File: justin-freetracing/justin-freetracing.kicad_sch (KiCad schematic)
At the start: 114 parts, among them J1 Conn_01x08_MountingPin, J2 Conn_02x03_Odd_Even, J3 Conn_01x08_MountingPin, J5 Barrel_Jack_Switch_Pin3Ring, K1 SW_Push, K10 SW_Push, K11 SW_Push, K12 SW_Push, K13 SW_Push, K14 SW_Push, K15 SW_Push, K16 SW_Push, K17 SW_Push, K18 SW_Push, K19 SW_Push, K2 SW_Push, K20 SW_Push, K21 SW_Push, K22 SW_Push, K23 SW_Push, K24 SW_Push, K25 SW_Push, K26 SW_Push, K27 SW_Push, K28 SW_Push, K29 SW_Push, K3 SW_Push, K30 SW_Push, K31 SW_Push, K32 SW_Push, K33 SW_Push, K34 SW_Push, K35 SW_Push, K36 SW_Push, K37 SW_Push, K38 SW_Push, K39 SW_Push, K4 SW_Push, K40 SW_Push, K41 SW_Push, K42 SW_Push, K43 SW_Push, K44 SW_Push, K45 SW_Push, K46 SW_Push, K47 SW_Push, K48 SW_Push, K49 SW_Push, K5 SW_Push, K6 SW_Push, K7 SW_Push, K8 SW_Push, K9 SW_Push, U1 ATmega1284-P, Y1 20MHz

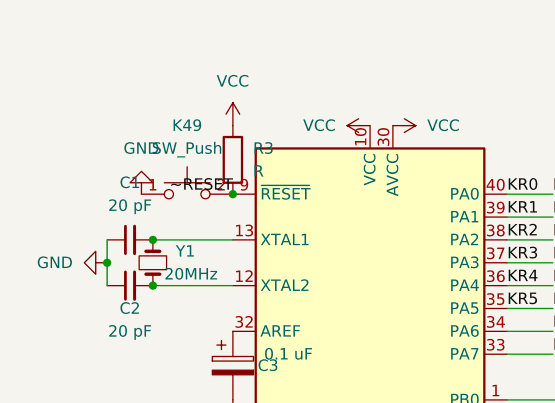
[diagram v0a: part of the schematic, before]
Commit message: Push
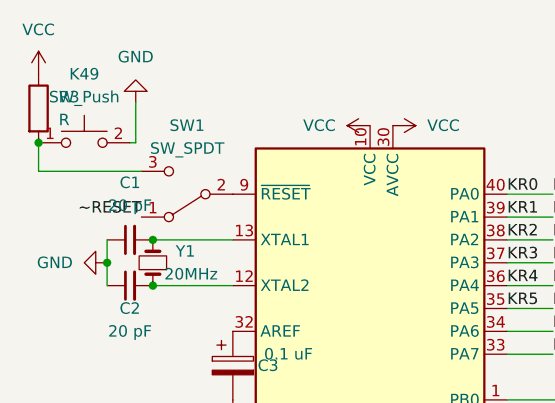
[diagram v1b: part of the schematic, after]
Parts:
- added SW1: SW_SPDT, Connector_PinSocket_2.54mm:PinSocket_1x03_P2.54mm_Vertical, symbol Switch:SW_SPDT
- R1, R2, R3: footprint Resistor_THT:R_Axial_DIN0204_L3.6mm_D1.6mm_P5.08mm_Horizontal -> Resistor_THT:R_Axial_DIN0204_L3.6mm_D1.6mm_P7.62mm_Horizontal
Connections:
- net GND: now also K49.2; no longer K49.1
- net ~RESET: now also SW1.1 (A); no longer K49.2, R3.2, U1.9 (~{RESET})
- new net: SW1.2 (B), U1.9 (~{RESET})
- new net: K49.1, R3.2, SW1.3 (C)
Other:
- moved on the sheet: K49, R3
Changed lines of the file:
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@@
   (junction (at 172.72 66.04) (diameter 0) (color 0 0 0 0)
   )
+  (junction (at 15.24 20.955) (diameter 0) (color 0 0 0 0)
+  )
   (junction (at 209.55 81.28) (diameter 0) (color 0 0 0 0)
   )
@@
   (junction (at 153.67 128.27) (diameter 0) (color 0 0 0 0)
   )
-  (junction (at 36.83 26.67) (diameter 0) (color 0 0 0 0)
-  )
   (junction (at 153.67 102.87) (diameter 0) (color 0 0 0 0)
   )
@@
     (stroke (width 0) (type default) (color 0 0 0 0))
   )
+  (wire (pts (xy 15.24 24.13) (xy 26.67 24.13))
+    (stroke (width 0) (type default) (color 0 0 0 0))
+  )
   (wire (pts (xy 144.78 68.58) (xy 152.4 68.58))
     (stroke (width 0) (type default) (color 0 0 0 0))
@@
     (stroke (width 0) (type default) (color 0 0 0 0))
   )
+  (wire (pts (xy 26.035 20.955) (xy 26.035 16.51))
+    (stroke (width 0) (type default) (color 0 0 0 0))
+  )
   (wire (pts (xy 67.31 41.91) (xy 72.39 41.91))
     (stroke (width 0) (type default) (color 0 0 0 0))
@@
     (stroke (width 0) (type default) (color 0 0 0 0))
   )
+  (wire (pts (xy 15.24 20.955) (xy 15.24 24.13))
+    (stroke (width 0) (type default) (color 0 0 0 0))
+  )
   (wire (pts (xy 134.62 88.9) (xy 134.62 90.17))
     (stroke (width 0) (type default) (color 0 0 0 0))
@@
     (stroke (width 0) (type default) (color 0 0 0 0))
   )
+  (wire (pts (xy 25.4 20.955) (xy 26.035 20.955))
+    (stroke (width 0) (type default) (color 0 0 0 0))
+  )
   (wire (pts (xy 144.78 81.28) (xy 152.4 81.28))
     (stroke (width 0) (type default) (color 0 0 0 0))
@@
     (effects (font (size 1.27 1.27)) (justify left bottom))
   )
-  (label "~RESET" (at 36.83 26.67 180)
+  (label "~RESET" (at 26.67 29.21 180)
     (effects (font (size 1.27 1.27)) (justify right bottom))
   )
@@
     (pin "2")
   )
+  (symbol (lib_id "Switch:SW_SPDT") (at 31.75 26.67 180) (unit 1)
+    (in_bom yes) (on_board yes) (fields_autoplaced)
+    (property "Reference" "SW1" (id 0) (at 31.75 19.05 0))
+    (property "Value" "SW_SPDT" (id 1) (at 31.75 21.59 0))
+    (property "Footprint" "Connector_PinSocket_2.54mm:PinSocket_1x03_P2.54mm_Vertical" (id 2) (at 31.75 26.67 0)
+      (effects (font (size 1.27 1.27)) hide)
+    )
+    (property "Datasheet" "~" (id 3) (at 31.75 26.67 0)
+      (effects (font (size 1.27 1.27)) hide)
+    )
+    (pin "1")
+    (pin "2")
+    (pin "3")
+  )
   (symbol (lib_id "Switch:SW_Push") (at 120.65 76.2 0) (unit 1)
     (in_bom yes) (on_board yes) (fields_autoplaced)
@@
     (pin "2")
   )
-  (symbol (lib_id "power:VCC") (at 36.83 19.05 0) (unit 1)
+  (symbol (lib_id "power:VCC") (at 15.24 13.335 0) (unit 1)
     (in_bom yes) (on_board yes) (fields_autoplaced)
-    (property "Reference" "#PWR0117" (id 0) (at 36.83 22.86 0)
+    (property "Reference" "#PWR0117" (id 0) (at 15.24 17.145 0)
       (effects (font (size 1.27 1.27)) hide)
     )
-    (property "Value" "VCC" (id 1) (at 36.83 14.1224 0))
-    (property "Footprint" "" (id 2) (at 36.83 19.05 0)
+    (property "Value" "VCC" (id 1) (at 15.24 8.4074 0))
+    (property "Footprint" "" (id 2) (at 15.24 13.335 0)
       (effects (font (size 1.27 1.27)) hide)
     )
-    (property "Datasheet" "" (id 3) (at 36.83 19.05 0)
+    (property "Datasheet" "" (id 3) (at 15.24 13.335 0)
       (effects (font (size 1.27 1.27)) hide)
     )
@@
       (effects (font (size 1.27 1.27)) (justify left))
     )
-    (property "Footprint" "Resistor_THT:R_Axial_DIN0204_L3.6mm_D1.6mm_P5.08mm_Horizontal" (id 2) (at 166.3192 17.8308 90)
+    (property "Footprint" "Resistor_THT:R_Axial_DIN0204_L3.6mm_D1.6mm_P7.62mm_Horizontal" (id 2) (at 166.3192 17.8308 90)
       (effects (font (size 1.27 1.27)) hide)
     )
@@
     (pin "2")
   )
-  (symbol (lib_id "power:GND") (at 26.67 26.67 180) (unit 1)
+  (symbol (lib_id "power:GND") (at 26.035 16.51 180) (unit 1)
     (in_bom yes) (on_board yes) (fields_autoplaced)
-    (property "Reference" "#PWR0118" (id 0) (at 26.67 20.32 0)
+    (property "Reference" "#PWR0118" (id 0) (at 26.035 10.16 0)
       (effects (font (size 1.27 1.27)) hide)
     )
-    (property "Value" "GND" (id 1) (at 26.67 21.59 0))
-    (property "Footprint" "" (id 2) (at 26.67 26.67 0)
+    (property "Value" "GND" (id 1) (at 26.035 11.43 0))
+    (property "Footprint" "" (id 2) (at 26.035 16.51 0)
       (effects (font (size 1.27 1.27)) hide)
     )
-    (property "Datasheet" "" (id 3) (at 26.67 26.67 0)
+    (property "Datasheet" "" (id 3) (at 26.035 16.51 0)
       (effects (font (size 1.27 1.27)) hide)
     )
@@
       (effects (font (size 1.27 1.27)) (justify left))
     )
-    (property "Footprint" "Resistor_THT:R_Axial_DIN0204_L3.6mm_D1.6mm_P5.08mm_Horizontal" (id 2) (at 157.6832 17.9832 90)
+    (property "Footprint" "Resistor_THT:R_Axial_DIN0204_L3.6mm_D1.6mm_P7.62mm_Horizontal" (id 2) (at 157.6832 17.9832 90)
       (effects (font (size 1.27 1.27)) hide)
     )
@@
     (pin "1")
   )
-  (symbol (lib_name "SW_Push_1") (lib_id "Switch:SW_Push") (at 31.75 26.67 0) (unit 1)
+  (symbol (lib_name "SW_Push_1") (lib_id "Switch:SW_Push") (at 20.32 20.955 0) (unit 1)
     (in_bom yes) (on_board yes)
-    (property "Reference" "K49" (id 0) (at 31.75 19.05 0))
-    (property "Value" "SW_Push" (id 1) (at 31.75 21.59 0))
-    (property "Footprint" "Button_Switch_Keyboard:SW_Cherry_MX_1.00u_PCB" (id 2) (at 31.75 21.59 0)
+    (property "Reference" "K49" (id 0) (at 20.32 13.335 0))
+    (property "Value" "SW_Push" (id 1) (at 20.32 15.875 0))
+    (property "Footprint" "Button_Switch_Keyboard:SW_Cherry_MX_1.00u_PCB" (id 2) (at 20.32 15.875 0)
       (effects (font (size 1.27 1.27)) hide)
     )
-    (property "Datasheet" "~" (id 3) (at 31.75 21.59 0)
+    (property "Datasheet" "~" (id 3) (at 20.32 15.875 0)
       (effects (font (size 1.27 1.27)) hide)
     )
@@
     (pin "2")
   )
-  (symbol (lib_id "Device:R") (at 36.83 22.86 0) (unit 1)
+  (symbol (lib_id "Device:R") (at 15.24 17.145 0) (unit 1)
     (in_bom yes) (on_board yes) (fields_autoplaced)
-    (property "Reference" "R3" (id 0) (at 39.0652 21.5899 0)
+    (property "Reference" "R3" (id 0) (at 17.4752 15.8749 0)
       (effects (font (size 1.27 1.27)) (justify left))
     )
-    (property "Value" "R" (id 1) (at 39.0652 24.1299 0)
+    (property "Value" "R" (id 1) (at 17.4752 18.4149 0)
       (effects (font (size 1.27 1.27)) (justify left))
     )
-    (property "Footprint" "Resistor_THT:R_Axial_DIN0204_L3.6mm_D1.6mm_P5.08mm_Horizontal" (id 2) (at 35.052 22.86 90)
+    (property "Footprint" "Resistor_THT:R_Axial_DIN0204_L3.6mm_D1.6mm_P7.62mm_Horizontal" (id 2) (at 13.462 17.145 90)
       (effects (font (size 1.27 1.27)) hide)
     )
-    (property "Datasheet" "~" (id 3) (at 36.83 22.86 0)
+    (property "Datasheet" "~" (id 3) (at 15.24 17.145 0)
       (effects (font (size 1.27 1.27)) hide)
     )
@@
     )
     (path "/ef34c09e-65f0-4b13-841b-8f0b0585a46d"
-      (reference "R1") (unit 1) (value "R") (footprint "Resistor_THT:R_Axial_DIN0204_L3.6mm_D1.6mm_P5.08mm_Horizontal")
+      (reference "R1") (unit 1) (value "R") (footprint "Resistor_THT:R_Axial_DIN0204_L3.6mm_D1.6mm_P7.62mm_Horizontal")
     )
     (path "/5a02d18b-6334-416e-a527-4bd7d2d39801"
-      (reference "R2") (unit 1) (value "R") (footprint "Resistor_THT:R_Axial_DIN0204_L3.6mm_D1.6mm_P5.08mm_Horizontal")
+      (reference "R2") (unit 1) (value "R") (footprint "Resistor_THT:R_Axial_DIN0204_L3.6mm_D1.6mm_P7.62mm_Horizontal")
     )
     (path "/f7b7181f-cee6-4f99-b51d-6e81e321ed3a"
-      (reference "R3") (unit 1) (value "R") (footprint "Resistor_THT:R_Axial_DIN0204_L3.6mm_D1.6mm_P5.08mm_Horizontal")
+      (reference "R3") (unit 1) (value "R") (footprint "Resistor_THT:R_Axial_DIN0204_L3.6mm_D1.6mm_P7.62mm_Horizontal")
+    )
+    (path "/1516ba09-5399-45fa-a362-0797687779e6"
+      (reference "SW1") (unit 1) (value "SW_SPDT") (footprint "Connector_PinSocket_2.54mm:PinSocket_1x03_P2.54mm_Vertical")
     )
     (path "/2cb05d43-df82-498c-aae1-4b1a0a350f82"
